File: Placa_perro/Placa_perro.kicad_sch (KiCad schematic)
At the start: 34 parts, among them J1 S_TEMPERATURA, J11 PANTALLA, J12 ENTRADA, J13 OPTO, J14 SALIDA_3.3v, J16 12v, J17 5v, J18 3.3v, J19 GND, J2 LDR, J20 LDR, J22 SALIDA_RELE_1, J4 S_GAS1, J5 S_GAS2, J6 USB_B, J8 Placa control, K2 Relay_SPDT, Q2 BC337, SW1 SW_DPDT_x2, U1 ESP32-Devkit-V1, U2 LM7805_TO220, U3 PC817

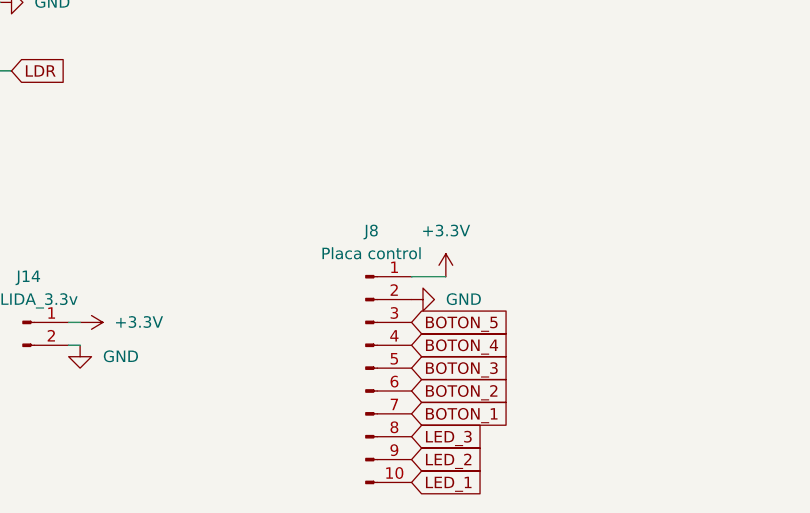
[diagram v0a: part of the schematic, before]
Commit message: terminada
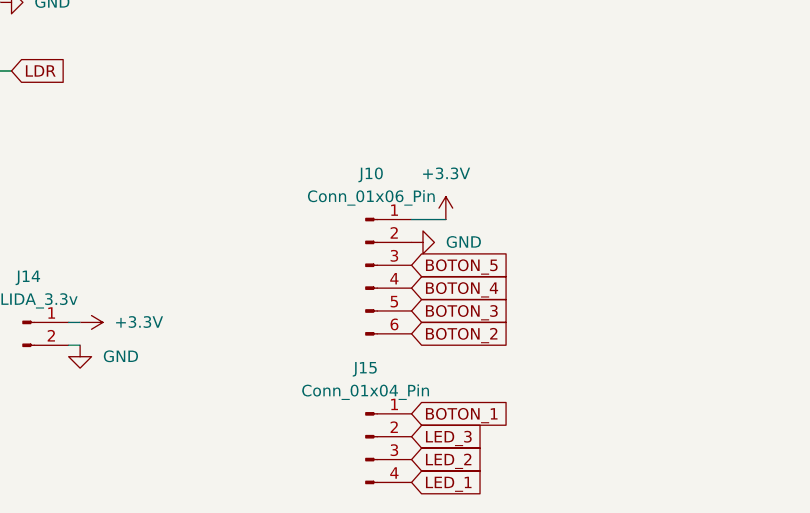
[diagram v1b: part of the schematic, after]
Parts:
- removed J8: Placa control, Connector_PinHeader_2.54mm:PinHeader_1x10_P2.54mm_Vertical, symbol Connector:Conn_01x10_Pin
- added J10: Conn_01x06_Pin, Connector_Molex:Molex_KK-254_AE-6410-06A_1x06_P2.54mm_Vertical, symbol Connector:Conn_01x06_Pin
- added J15: Conn_01x04_Pin, Connector_Molex:Molex_KK-254_AE-6410-04A_1x04_P2.54mm_Vertical, symbol Connector:Conn_01x04_Pin
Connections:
- net +3.3V: now also J10.1 (Pin_1)
- net BOTON_1: now also J15.1 (Pin_1)
- net BOTON_2: now also J10.6 (Pin_6)
- net BOTON_3: now also J10.5 (Pin_5)
- net BOTON_4: now also J10.4 (Pin_4)
- net BOTON_5: now also J10.3 (Pin_3)
- net GND: now also J10.2 (Pin_2)
- net LED_1: now also J15.4 (Pin_4)
- net LED_2: now also J15.3 (Pin_3)
- net LED_3: now also J15.2 (Pin_2)
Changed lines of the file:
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@@
 	(wire
 		(pts
-			(xy 76.2 168.91) (xy 80.01 168.91)
+			(xy 76.2 162.56) (xy 80.01 162.56)
 		)
 		(stroke
@@
 	(global_label "BOTON_5"
 		(shape input)
-		(at 76.2 173.99 0)
+		(at 76.2 167.64 0)
 		(fields_autoplaced yes)
 		(effects
@@
 		)
 		(property "Intersheetrefs" "${INTERSHEET_REFS}"
-			(at 87.5914 173.99 0)
+			(at 87.5914 167.64 0)
 			(effects
 				(font
@@
 	(global_label "BOTON_3"
 		(shape input)
-		(at 76.2 179.07 0)
+		(at 76.2 172.72 0)
 		(fields_autoplaced yes)
 		(effects
@@
 		)
 		(property "Intersheetrefs" "${INTERSHEET_REFS}"
-			(at 87.5914 179.07 0)
+			(at 87.5914 172.72 0)
 			(effects
 				(font
@@
 	(global_label "BOTON_2"
 		(shape input)
-		(at 76.2 181.61 0)
+		(at 76.2 175.26 0)
 		(fields_autoplaced yes)
 		(effects
@@
 		)
 		(property "Intersheetrefs" "${INTERSHEET_REFS}"
-			(at 87.5914 181.61 0)
+			(at 87.5914 175.26 0)
 			(effects
 				(font
@@
 	(global_label "BOTON_4"
 		(shape input)
-		(at 76.2 176.53 0)
+		(at 76.2 170.18 0)
 		(fields_autoplaced yes)
 		(effects
@@
 		)
 		(property "Intersheetrefs" "${INTERSHEET_REFS}"
-			(at 87.5914 176.53 0)
+			(at 87.5914 170.18 0)
 			(effects
 				(font
@@
 	(symbol
 		(lib_id "power:+3.3V")
-		(at 80.01 168.91 0)
+		(at 80.01 162.56 0)
 		(unit 1)
 		(exclude_from_sim no)
@@
 		(fields_autoplaced yes)
 		(property "Reference" "#PWR059"
-			(at 80.01 172.72 0)
+			(at 80.01 166.37 0)
 			(effects
 				(font
@@
 		)
 		(property "Value" "+3.3V"
-			(at 80.01 163.83 0)
+			(at 80.01 157.48 0)
 			(effects
 				(font
@@
 		)
 		(property "Footprint" ""
-			(at 80.01 168.91 0)
+			(at 80.01 162.56 0)
 			(effects
 				(font
@@
 		)
 		(property "Datasheet" ""
-			(at 80.01 168.91 0)
+			(at 80.01 162.56 0)
 			(effects
 				(font
@@
 		)
 		(property "Description" "Power symbol creates a global label with name \"+3.3V\""
-			(at 80.01 168.91 0)
+			(at 80.01 162.56 0)
 			(effects
 				(font
@@
 	)
 	(symbol
+		(lib_id "Connector:Conn_01x06_Pin")
+		(at 71.12 167.64 0)
+		(unit 1)
+		(exclude_from_sim no)
+		(in_bom yes)
+		(on_board yes)
+		(dnp no)
+		(fields_autoplaced yes)
+		(property "Reference" "J10"
+			(at 71.755 157.48 0)
+			(effects
+				(font
+					(size 1.27 1.27)
+				)
+			)
+		)
+		(property "Value" "Conn_01x06_Pin"
+			(at 71.755 160.02 0)
+			(effects
+				(font
+					(size 1.27 1.27)
+				)
+			)
+		)
+		(property "Footprint" "Connector_Molex:Molex_KK-254_AE-6410-06A_1x06_P2.54mm_Vertical"
+			(at 71.12 167.64 0)
+			(effects
+				(font
+					(size 1.27 1.27)
+				)
+				(hide yes)
+			)
+		)
+		(property "Datasheet" "~"
+			(at 71.12 167.64 0)
+			(effects
+				(font
+					(size 1.27 1.27)
+				)
+				(hide yes)
+			)
+		)
+		(property "Description" "Generic connector, single row, 01x06, script generated"
+			(at 71.12 167.64 0)
+			(effects
+				(font
+					(size 1.27 1.27)
+				)
+				(hide yes)
+			)
+		)
+		(pin "3"
+		)
+		(pin "6"
+		)
+		(pin "1"
+		)
+		(pin "5"
+		)
+		(pin "2"
+		)
+		(pin "4"
+		)
+		(instances
+			(project ""
+				(path "/65c2dfe9-d457-45cc-a8ad-62a01e187037"
+					(reference "J10")
+					(unit 1)
+				)
+			)
+		)
+	)
+	(symbol
 		(lib_id "Connector:Conn_01x01_Pin")
 		(at 24.13 123.19 0)
@@
 	)
 	(symbol
+		(lib_id "Connector:Conn_01x04_Pin")
+		(at 71.12 186.69 0)
+		(unit 1)
+		(exclude_from_sim no)
+		(in_bom yes)
+		(on_board yes)
+		(dnp no)
+		(property "Reference" "J15"
+			(at 71.12 179.07 0)
+			(effects
+				(font
+					(size 1.27 1.27)
+				)
+			)
+		)
+		(property "Value" "Conn_01x04_Pin"
+			(at 71.12 181.61 0)
+			(effects
+				(font
+					(size 1.27 1.27)
+				)
+			)
+		)
+		(property "Footprint" "Connector_Molex:Molex_KK-254_AE-6410-04A_1x04_P2.54mm_Vertical"
+			(at 71.12 186.69 0)
+			(effects
+				(font
+					(size 1.27 1.27)
+				)
+				(hide yes)
+			)
+		)
+		(property "Datasheet" "~"
+			(at 71.12 186.69 0)
+			(effects
+				(font
+					(size 1.27 1.27)
+				)
+				(hide yes)
+			)
+		)
+		(property "Description" "Generic connector, single row, 01x04, script generated"
+			(at 71.12 186.69 0)
+			(effects
+				(font
+					(size 1.27 1.27)
+				)
+				(hide yes)
+			)
+		)
+		(pin "2"
+		)
+		(pin "3"
+		)
+		(pin "1"
+		)
+		(pin "4"
+		)
+		(instances
+			(project ""
+				(path "/65c2dfe9-d457-45cc-a8ad-62a01e187037"
+					(reference "J15")
+					(unit 1)
+				)
+			)
+		)
+	)
+	(symbol
 		(lib_id "power:GND")
 		(at 36.83 99.06 0)
@@
 	)
 	(symbol
-		(lib_id "Connector:Conn_01x10_Pin")
-		(at 71.12 179.07 0)
-		(unit 1)
-		(exclude_from_sim no)
-		(in_bom yes)
-		(on_board yes)
-		(dnp no)
-		(fields_autoplaced yes)
-		(property "Reference" "J8"
-			(at 71.755 163.83 0)
-			(effects
-				(font
-					(size 1.27 1.27)
-				)
-			)
-		)
-		(property "Value" "Placa control"
-			(at 71.755 166.37 0)
-			(effects
-				(font
-					(size 1.27 1.27)
-				)
-			)
-		)
-		(property "Footprint" "Connector_PinHeader_2.54mm:PinHeader_1x10_P2.54mm_Vertical"
-			(at 71.12 179.07 0)
-			(effects
-				(font
-					(size 1.27 1.27)
-				)
-				(hide yes)
-			)
-		)
-		(property "Datasheet" "~"
-			(at 71.12 179.07 0)
-			(effects
-				(font
-					(size 1.27 1.27)
-				)
-				(hide yes)
-			)
-		)
-		(property "Description" "Generic connector, single row, 01x10, script generated"
-			(at 71.12 179.07 0)
-			(effects
-				(font
-					(size 1.27 1.27)
-				)
-				(hide yes)
-			)
-		)
-		(pin "6"
-		)
-		(pin "5"
-		)
-		(pin "1"
-		)
-		(pin "2"
-		)
-		(pin "7"
-		)
-		(pin "8"
-		)
-		(pin "9"
-		)
-		(pin "10"
-		)
-		(pin "4"
-		)
-		(pin "3"
-		)
-		(instances
-			(project "Placa_perro"
-				(path "/65c2dfe9-d457-45cc-a8ad-62a01e187037"
-					(reference "J8")
-					(unit 1)
-				)
-			)
-		)
-	)
-	(symbol
 		(lib_id "Connector:Conn_01x02_Pin")
 		(at 16.51 24.13 0)
@@
 	(symbol
 		(lib_id "power:GND")
-		(at 76.2 171.45 90)
+		(at 76.2 165.1 90)
 		(unit 1)
 		(exclude_from_sim no)
@@
 		(fields_autoplaced yes)
 		(property "Reference" "#PWR015"
-			(at 82.55 171.45 0)
+			(at 82.55 165.1 0)
 			(effects
 				(font
@@
 		)
 		(property "Value" "GND"
-			(at 80.01 171.4499 90)
+			(at 80.01 165.0999 90)
 			(effects
 				(font
@@
 		)
 		(property "Footprint" ""
-			(at 76.2 171.45 0)
+			(at 76.2 165.1 0)
 			(effects
 				(font
@@
 		)
 		(property "Datasheet" ""
-			(at 76.2 171.45 0)
+			(at 76.2 165.1 0)
 			(effects
 				(font
@@
 		)
 		(property "Description" "Power symbol creates a global label with name \"GND\" , ground"
-			(at 76.2 171.45 0)
+			(at 76.2 165.1 0)
 			(effects
 				(font
